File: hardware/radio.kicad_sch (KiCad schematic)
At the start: 61 parts, among them J1 105450-0101, J2 Conn_01x02, J3 Conn_01x02, J4 Conn_01x04, J5 Conn_01x02_Male, Q1 Q_PMOS_DGS, Q2 Q_NMOS_DGS, Q3 Q_NMOS_DGS, Q4 Q_PMOS_DGS, SW1 SW_BOOT, SW2 SW_RST, SW3 SW_1, SW4 Rot_Enc, SW5 SW_2, SW6 SW_3, U1 TP4056, U2 ESP32-WROOM-32, U3 TPS5432, U4 MAX98357

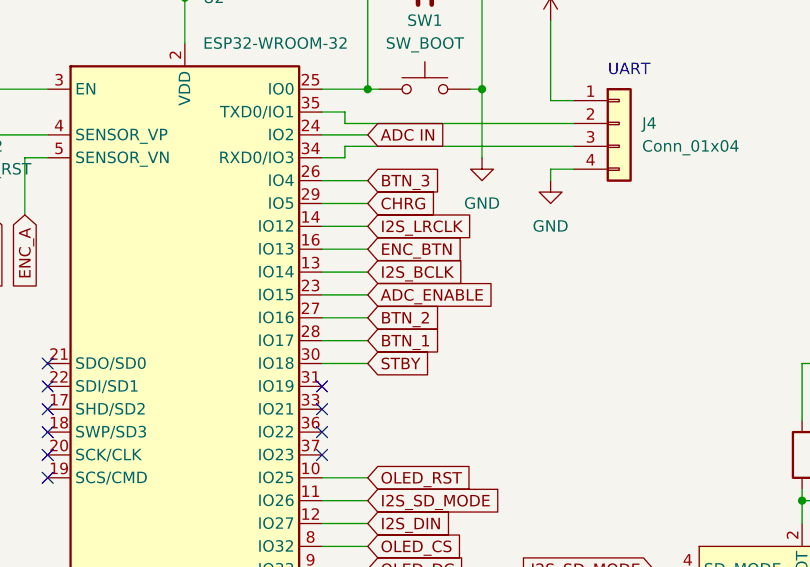
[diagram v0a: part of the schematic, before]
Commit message: routing
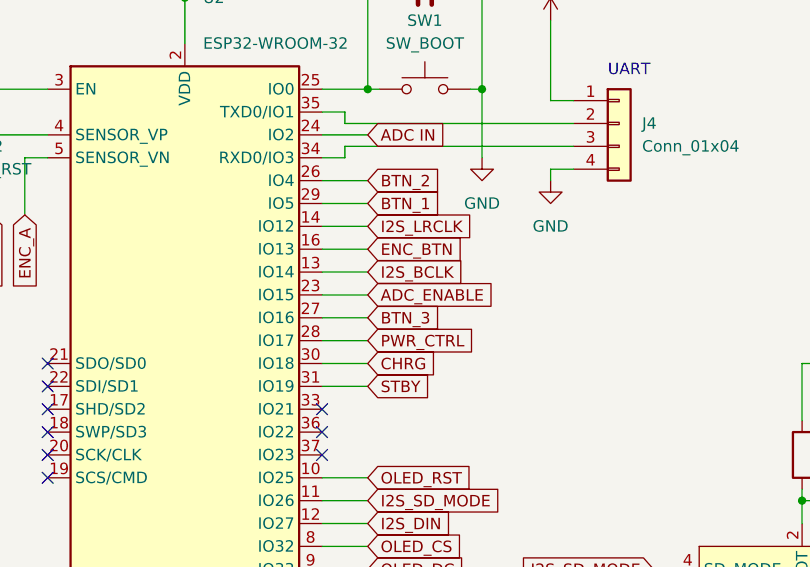
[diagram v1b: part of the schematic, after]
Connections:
- net BTN_1: now also U2.29 (IO5); no longer U2.28 (IO17)
- net BTN_2: now also U2.26 (IO4); no longer U2.27 (IO16)
- net BTN_3: now also U2.27 (IO16); no longer U2.26 (IO4)
- net CHRG: now also U2.30 (IO18); no longer U2.29 (IO5)
- net PWR_CTRL: now also U2.28 (IO17)
- net STBY: now also U2.31 (IO19); no longer U2.30 (IO18)
- no-connect marks 26 -> 25
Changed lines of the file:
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@@
   (no_connect (at 162.56 125.73))
   (no_connect (at 162.56 130.81))
-  (no_connect (at 162.56 123.19))
   (no_connect (at 25.4 93.98))
   (no_connect (at 25.4 83.82))
@@
     (stroke (width 0) (type default) (color 0 0 0 0))
   )
+  (wire (pts (xy 162.56 123.19) (xy 167.64 123.19))
+    (stroke (width 0) (type default) (color 0 0 0 0))
+  )
   (wire (pts (xy 115.57 154.94) (xy 115.57 153.67))
     (stroke (width 0) (type default) (color 0 0 0 0))
@@
     (effects (font (size 1.27 1.27)) (justify left bottom))
   )
-  (global_label "BTN_1" (shape input) (at 167.64 118.11 0) (fields_autoplaced)
-    (effects (font (size 1.27 1.27)) (justify left))
-    (property "Intersheet References" "${INTERSHEET_REFS}" (id 0) (at 175.7983 118.0306 0)
-      (effects (font (size 1.27 1.27)) (justify left) hide)
-    )
-  )
   (global_label "OLED_CLK" (shape input) (at 248.92 95.25 180) (fields_autoplaced)
     (effects (font (size 1.27 1.27)) (justify right))
@@
     )
   )
-  (global_label "BTN_2" (shape input) (at 167.64 115.57 0) (fields_autoplaced)
+  (global_label "BTN_3" (shape input) (at 167.64 115.57 0) (fields_autoplaced)
     (effects (font (size 1.27 1.27)) (justify left))
     (property "Intersheet References" "${INTERSHEET_REFS}" (id 0) (at 175.7983 115.4906 0)
@@
     )
   )
+  (global_label "BTN_1" (shape input) (at 167.64 102.87 0) (fields_autoplaced)
+    (effects (font (size 1.27 1.27)) (justify left))
+    (property "Intersheet References" "${INTERSHEET_REFS}" (id 0) (at 175.7983 102.7906 0)
+      (effects (font (size 1.27 1.27)) (justify left) hide)
+    )
+  )
   (global_label "I2S_SD_MODE" (shape input) (at 199.39 143.51 180) (fields_autoplaced)
     (effects (font (size 1.27 1.27)) (justify right))
@@
     )
   )
-  (global_label "STBY" (shape input) (at 167.64 120.65 0) (fields_autoplaced)
-    (effects (font (size 1.27 1.27)) (justify left))
-    (property "Intersheet References" "${INTERSHEET_REFS}" (id 0) (at 174.5888 120.5706 0)
+  (global_label "PWR_CTRL" (shape input) (at 167.64 118.11 0) (fields_autoplaced)
+    (effects (font (size 1.27 1.27)) (justify left))
+    (property "Intersheet References" "${INTERSHEET_REFS}" (id 0) (at 179.5479 118.0306 0)
       (effects (font (size 1.27 1.27)) (justify left) hide)
     )
@@
     )
   )
+  (global_label "BTN_2" (shape input) (at 167.64 100.33 0) (fields_autoplaced)
+    (effects (font (size 1.27 1.27)) (justify left))
+    (property "Intersheet References" "${INTERSHEET_REFS}" (id 0) (at 175.7983 100.2506 0)
+      (effects (font (size 1.27 1.27)) (justify left) hide)
+    )
+  )
+  (global_label "CHRG" (shape input) (at 167.64 120.65 0) (fields_autoplaced)
+    (effects (font (size 1.27 1.27)) (justify left))
+    (property "Intersheet References" "${INTERSHEET_REFS}" (id 0) (at 175.1936 120.5706 0)
+      (effects (font (size 1.27 1.27)) (justify left) hide)
+    )
+  )
   (global_label "ENC_A" (shape input) (at 129.54 104.14 270) (fields_autoplaced)
     (effects (font (size 1.27 1.27)) (justify right))
@@
     )
   )
-  (global_label "BTN_3" (shape input) (at 167.64 100.33 0) (fields_autoplaced)
-    (effects (font (size 1.27 1.27)) (justify left))
-    (property "Intersheet References" "${INTERSHEET_REFS}" (id 0) (at 175.7983 100.2506 0)
-      (effects (font (size 1.27 1.27)) (justify left) hide)
-    )
-  )
   (global_label "I2S_BCLK" (shape input) (at 167.64 110.49 0) (fields_autoplaced)
     (effects (font (size 1.27 1.27)) (justify left))
@@
     )
   )
-  (global_label "CHRG" (shape input) (at 167.64 102.87 0) (fields_autoplaced)
-    (effects (font (size 1.27 1.27)) (justify left))
-    (property "Intersheet References" "${INTERSHEET_REFS}" (id 0) (at 175.1936 102.7906 0)
-      (effects (font (size 1.27 1.27)) (justify left) hide)
-    )
-  )
   (global_label "ENC_S1" (shape input) (at 107.95 116.84 0) (fields_autoplaced)
     (effects (font (size 1.27 1.27)) (justify left))
@@
       (effects (font (size 1.27 1.27)) (justify left) hide)
     )
+  )
+  (global_label "STBY" (shape input) (at 167.64 123.19 0) (fields_autoplaced)
+    (effects (font (size 1.27 1.27)) (justify left))
+    (property "Intersheet References" "${INTERSHEET_REFS}" (id 0) (at 174.5888 123.1106 0)
+      (effects (font (size 1.27 1.27)) (justify left) hide)
+    )
